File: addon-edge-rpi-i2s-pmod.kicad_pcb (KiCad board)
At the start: 2 copper layers, 100 x 100 mm, 39 parts, among them J1 PMOD1, J10 Conn_01x02, J12 Conn_01x02, J13 Conn_01x01, J2 PMOD2, J3 PMOD3, J4 PMOD4, J5 Conn_01x06, J6 Conn_01x06, J7 Conn_01x03, J8 Conn_01x04, J9 Conn_01x05

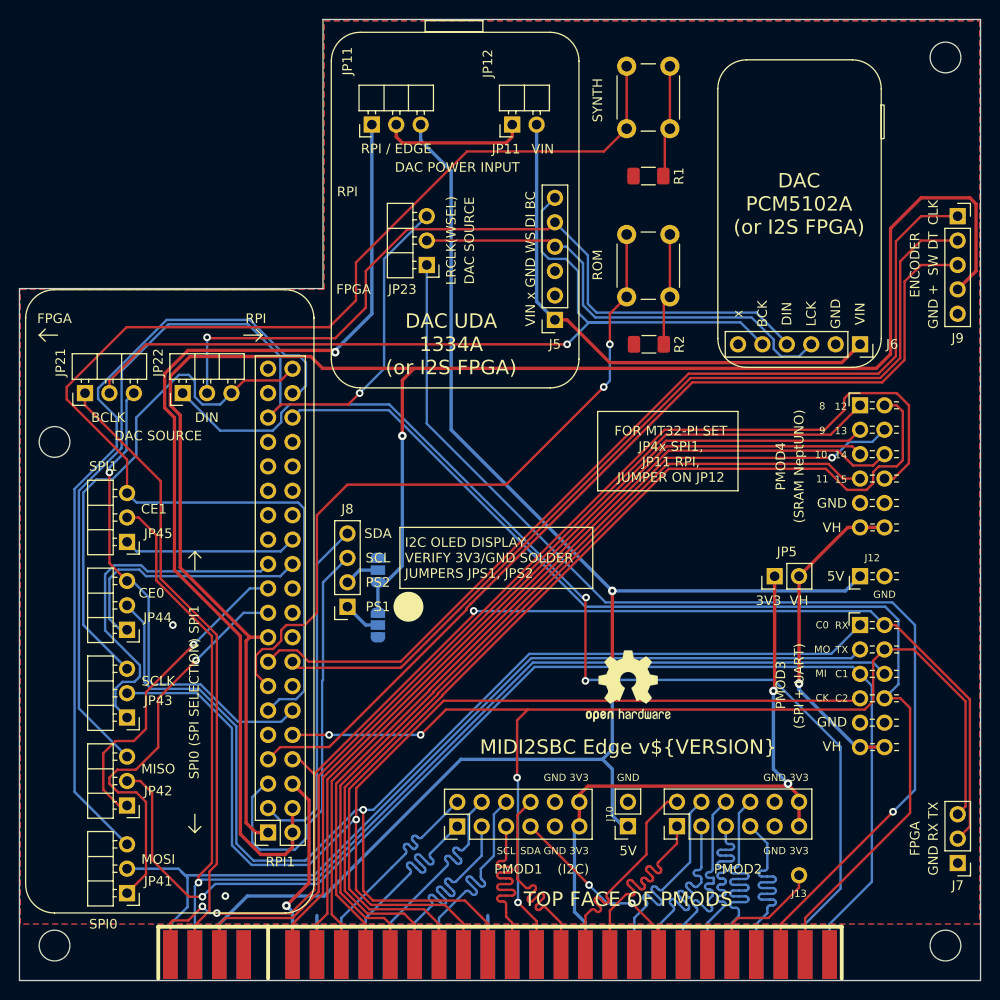
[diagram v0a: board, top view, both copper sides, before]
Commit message: v0.7 sent to manufacturing
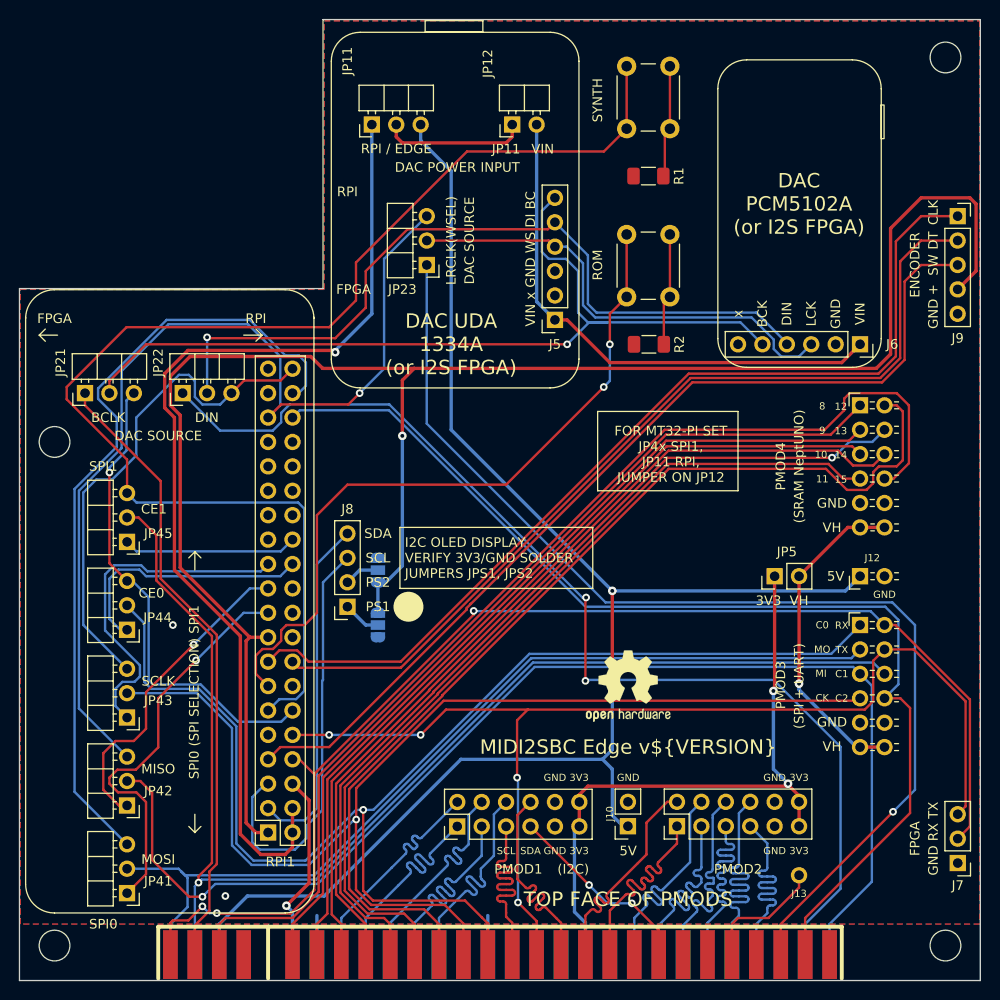
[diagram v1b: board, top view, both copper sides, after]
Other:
- board text added: "0.2000 mm / 0.2032 mm"
- board text added: "0.3000 mm"
- board text added: "1.6000 mm"
- board text added: "2"
- board text added: "99.9850 mm x 99.9990 mm"
- board text added: "BOARD CHARACTERISTICS"
- board text added: "Board Thickness:"
- board text added: "Board overall dimensions:"
- board text added: "Castellated pads:"
- board text added: "Copper Finish:"
- board text added: "Copper Layer Count:"
- board text added: "Edge card connectors:"
- board text added: "Impedance Control:"
- board text added: "Min hole diameter:"
- board text added: "Min track/spacing:"
- board text added: "No"
- board text added: "None"
- board text added: "Plated Board Edge:"
- board text added: "checklist: https://github.com/azonenberg/pcb-checklist/"
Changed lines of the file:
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@@
       (viasonmask false)
       (mode 1)
-      (useauxorigin true)
+      (useauxorigin false)
       (hpglpennumber 1)
       (hpglpenspeed 20)
@@
       (plotinvisibletext false)
       (sketchpadsonfab false)
-      (subtractmaskfromsilk false)
+      (subtractmaskfromsilk true)
       (outputformat 1)
       (mirror false)
@@
     )
   )
-  (property "VERSION" "0.6")
+  (property "VERSION" "0.7")
   (net 0 "")
   (net 1 "/B26_WSEL_LRCLK_I2S")
@@
   (gr_line (start 110.8075 77.7875) (end 111.4425 77.1525) (layer "F.SilkS") (width 0.12))
   (gr_line (start 110.8075 77.7875) (end 111.4425 78.4225) (layer "F.SilkS") (width 0.12))
-  (gr_line (start 208.75 44.9397) (end 208.75 144.93875) (layer "Edge.Cuts") (width 0.05))
-  (gr_line (start 140.335 44.9397) (end 208.75 44.9397) (layer "Edge.Cuts") (width 0.05))
-  (gr_line (start 108.75 144.93875) (end 208.75 144.93875) (layer "Edge.Cuts") (width 0.05))
-  (gr_line (start 140.335 72.9387) (end 140.335 44.9397) (layer "Edge.Cuts") (width 0.05))
-  (gr_line (start 108.75 144.93875) (end 108.75 72.9387) (layer "Edge.Cuts") (width 0.05))
-  (gr_line (start 108.75 72.9387) (end 140.335 72.9387) (layer "Edge.Cuts") (width 0.05))
+  (gr_line (start 208.725 44.9497) (end 208.725 144.93875) (layer "Edge.Cuts") (width 0.01))
+  (gr_line (start 140.335 44.9497) (end 208.725 44.9497) (layer "Edge.Cuts") (width 0.01))
+  (gr_line (start 108.75 144.93875) (end 208.725 144.93875) (layer "Edge.Cuts") (width 0.01))
+  (gr_line (start 140.335 72.9387) (end 140.335 44.9497) (layer "Edge.Cuts") (width 0.01))
+  (gr_line (start 108.75 144.93875) (end 108.75 72.9387) (layer "Edge.Cuts") (width 0.01))
+  (gr_line (start 108.75 72.9387) (end 140.335 72.9387) (layer "Edge.Cuts") (width 0.01))
   (gr_text "MIDI I2S SBC Pmod\nEdge Interface v${VERSION}\n\n" (at 167.64 119.38) (layer "B.SilkS")
     (effects (font (size 1.5 1.5) (thickness 0.15)) (justify mirror))
@@
     (effects (font (size 0.75 0.75) (thickness 0.15)))
   )
+  (gr_text "checklist: https://github.com/azonenberg/pcb-checklist/" (at 149.72 217.62) (layer "User.1")
+    (effects (font (size 3 3) (thickness 0.15)))
+  )
+  (gr_text "0.2000 mm / 0.2032 mm" (at 57.387143 44.98) (layer "User.1")
+    (effects (font (size 1.5 1.5) (thickness 0.2)) (justify left top))
+  )
+  (gr_text "Board Thickness: " (at 91.444286 35.95) (layer "User.1")
+    (effects (font (size 1.5 1.5) (thickness 0.2)) (justify left top))
+  )
+  (gr_text "Board overall dimensions: " (at 24.83 40.465) (layer "User.1")
+    (effects (font (size 1.5 1.5) (thickness 0.2)) (justify left top))
+  )
+  (gr_text "None" (at 57.387143 49.495) (layer "User.1")
+    (effects (font (size 1.5 1.5) (thickness 0.2)) (justify left top))
+  )
+  (gr_text "Castellated pads: " (at 24.83 54.01) (layer "User.1")
+    (effects (font (size 1.5 1.5) (thickness 0.2)) (justify left top))
+  )
+  (gr_text "Edge card connectors: " (at 24.83 58.525) (layer "User.1")
+    (effects (font (size 1.5 1.5) (thickness 0.2)) (justify left top))
+  )
+  (gr_text "No" (at 57.387143 58.525) (layer "User.1")
+    (effects (font (size 1.5 1.5) (thickness 0.2)) (justify left top))
+  )
+  (gr_text "0.3000 mm" (at 116.287143 44.98) (layer "User.1")
+    (effects (font (size 1.5 1.5) (thickness 0.2)) (justify left top))
+  )
+  (gr_text "99.9850 mm x 99.9990 mm" (at 57.387143 40.465) (layer "User.1")
+    (effects (font (size 1.5 1.5) (thickness 0.2)) (justify left top))
+  )
+  (gr_text "" (at 116.287143 40.465) (layer "User.1")
+    (effects (font (size 1.5 1.5) (thickness 0.2)) (justify left top))
+  )
+  (gr_text "Impedance Control: " (at 91.444286 49.495) (layer "User.1")
+    (effects (font (size 1.5 1.5) (thickness 0.2)) (justify left top))
+  )
+  (gr_text "No" (at 57.387143 54.01) (layer "User.1")
+    (effects (font (size 1.5 1.5) (thickness 0.2)) (justify left top))
+  )
+  (gr_text "Min hole diameter: " (at 91.444286 44.98) (layer "User.1")
+    (effects (font (size 1.5 1.5) (thickness 0.2)) (justify left top))
+  )
+  (gr_text "BOARD CHARACTERISTICS" (at 24.08 29.78) (layer "User.1")
+    (effects (font (size 2 2) (thickness 0.4)) (justify left top))
+  )
+  (gr_text "No" (at 116.287143 54.01) (layer "User.1")
+    (effects (font (size 1.5 1.5) (thickness 0.2)) (justify left top))
+  )
+  (gr_text "Min track/spacing: " (at 24.83 44.98) (layer "User.1")
+    (effects (font (size 1.5 1.5) (thickness 0.2)) (justify left top))
+  )
+  (gr_text "Plated Board Edge: " (at 91.444286 54.01) (layer "User.1")
+    (effects (font (size 1.5 1.5) (thickness 0.2)) (justify left top))
+  )
+  (gr_text "Copper Layer Count: " (at 24.83 35.95) (layer "User.1")
+    (effects (font (size 1.5 1.5) (thickness 0.2)) (justify left top))
+  )
+  (gr_text "No" (at 116.287143 49.495) (layer "User.1")
+    (effects (font (size 1.5 1.5) (thickness 0.2)) (justify left top))
+  )
+  (gr_text "2" (at 57.387143 35.95) (layer "User.1")
+    (effects (font (size 1.5 1.5) (thickness 0.2)) (justify left top))
+  )
+  (gr_text "1.6000 mm" (at 116.287143 35.95) (layer "User.1")
+    (effects (font (size 1.5 1.5) (thickness 0.2)) (justify left top))
+  )
+  (gr_text "Copper Finish: " (at 24.83 49.495) (layer "User.1")
+    (effects (font (size 1.5 1.5) (thickness 0.2)) (justify left top))
+  )
+  (gr_text "" (at 91.444286 40.465) (layer "User.1")
+    (effects (font (size 1.5 1.5) (thickness 0.2)) (justify left top))
+  )
   (dimension (type aligned) (layer "Dwgs.User")
-    (pts (xy 208.75 44.9397) (xy 208.75 144.93875))
+    (pts (xy 208.725 44.9497) (xy 208.725 144.93875))
     (height -10.96)
-    (gr_text "99.9990 mm" (at 217.805 94.615 90) (layer "Dwgs.User")
+    (gr_text "99.9891 mm" (at 217.805 94.615 90) (layer "Dwgs.User")
       (effects (font (size 1 1) (thickness 0.15)))
     )
@@
   )
   (dimension (type aligned) (layer "Dwgs.User")
-    (pts (xy 108.75 144.93875) (xy 208.75 144.93875))
+    (pts (xy 108.75 144.93875) (xy 208.725 144.93875))
     (height 9.36625)
-    (gr_text "100.0000 mm" (at 159.385 152.4) (layer "Dwgs.User")
+    (gr_text "99.9750 mm" (at 159.385 152.4) (layer "Dwgs.User")
       (effects (font (size 1 1) (thickness 0.15)))
     )
@@
     )
   )
+  (group "group-boardCharacteristics" (id 34b6b129-a76c-4a62-91cc-2743f5f4b2c4)
+    (members
+      4f0ad253-6758-4fab-a304-5619bb190326
+      5d6cfde2-9586-45a3-9d7e-b9db5ad7bc21
+      62cf0a26-9096-4000-923a-60daf3aa23f8
+      63777433-96ab-4b15-8870-c77f38cbb556
+      70e18146-fcad-491b-ae29-6b6b530cc027
+      738c73ca-416f-4cdc-b135-180d4d696484
+      7590e24b-577c-4fcd-9e1f-ab45b189df19
+      7cea007c-3280-4e58-94e8-fd0f1c985899
+      7f04153d-9d5e-47af-b99d-bc6a387c9a6f
+      897136b5-a5d5-4581-a6bf-48c25cde5ca5
+      8a80af2d-ce13-4b11-8a6d-9856813678bd
+      9b86d498-b713-4140-97c2-940c95f43f16
+      9fd2c636-f5cd-47e5-bbbc-56f7c25ff6b0
+      c7daa16d-2cdc-48f9-84e1-6fd3b9ab8609
+      d32ff0d3-6db2-4544-ab69-6c0b14790da2
+      ddcc8852-5683-4366-8128-1d6ff0a98b06
+      e0fafb5a-7612-49f2-857e-07a48cf36c67
+      e2eaff9d-4c94-4311-bec0-a13146b760ca
+      e34767e1-a29c-42c3-8abb-ef0a479b6adf
+      e66cdece-4893-4be4-8985-52fc83792731
+      e997c615-0a9d-46fc-872f-6b2d14f01b36
+      ed15d2ab-884d-4309-8fc5-a20c99e91302
+      f5156e03-6da9-4205-8d49-0997e01031c7
+    )
+  )
